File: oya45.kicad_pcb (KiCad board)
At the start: 2 copper layers, 190.5 x 95.2 mm, 108 parts, among them U1 ProMicro

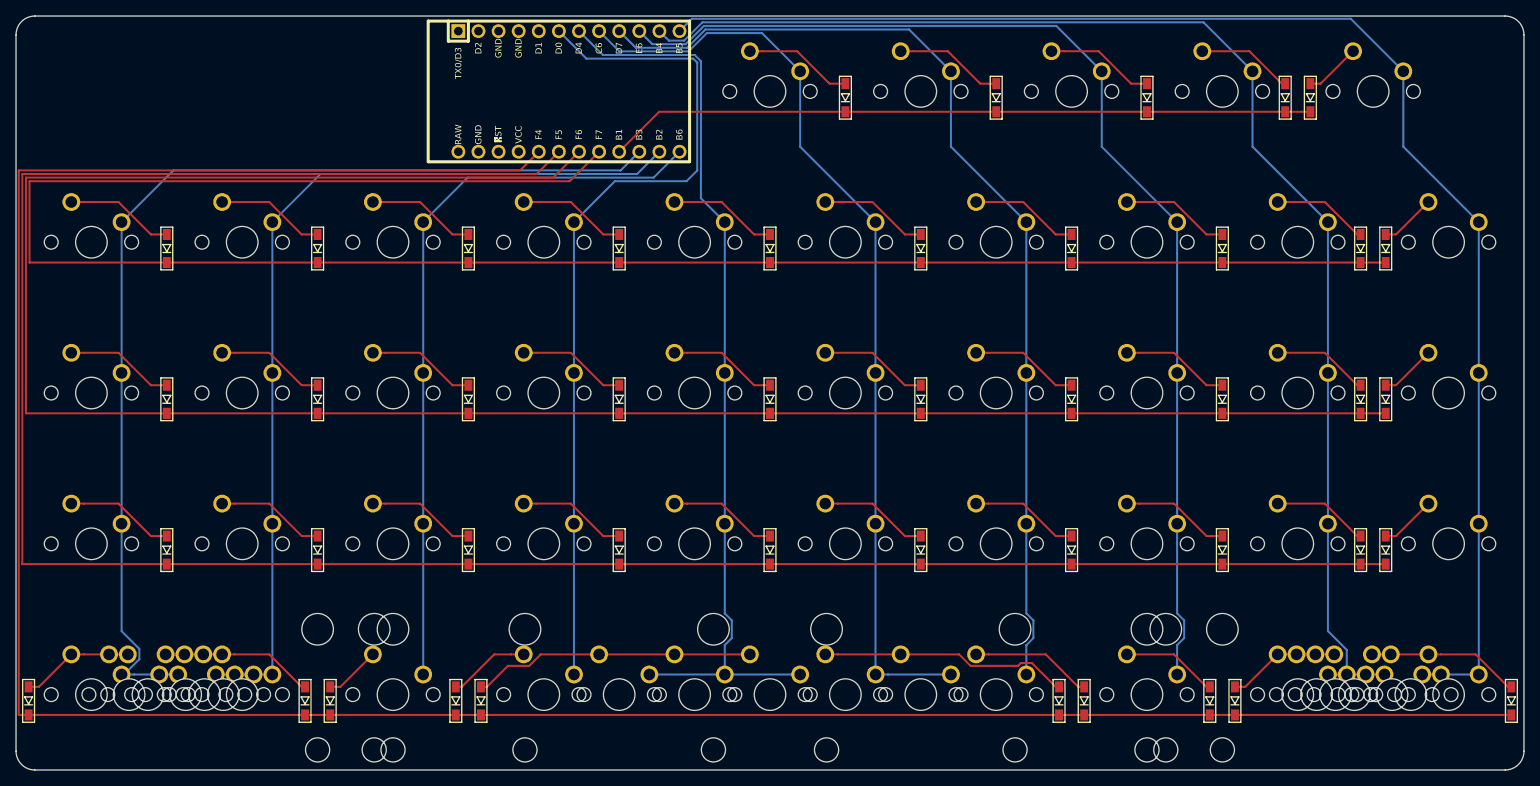
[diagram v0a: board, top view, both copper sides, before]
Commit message: added ground fill
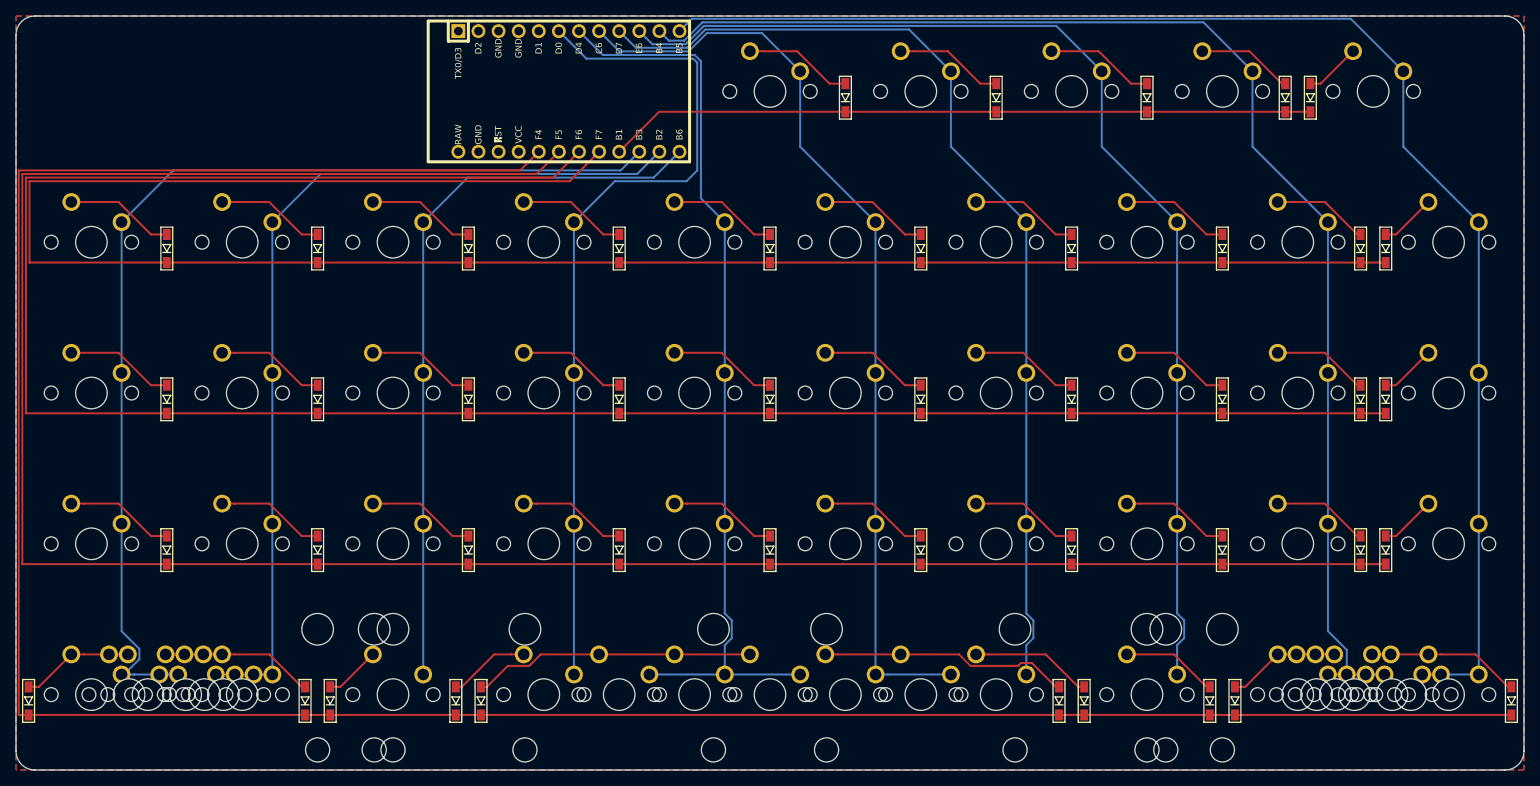
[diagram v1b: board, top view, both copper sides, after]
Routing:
- added copper zone on B.Cu, net (none)
- added copper zone on F.Cu, net (none)
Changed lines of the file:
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@@
   (segment (start 216.23974 28.91474) (end 133.01026 28.91474) (width 0.254) (layer B.Cu) (net 60))
   (segment (start 232.41 111.76) (end 225.26625 111.76) (width 0.254) (layer B.Cu) (net 60))
+  (zone (net 0) (net_name "") (layer F.Cu) (hatch edge 0.508)
+    (connect_pads (clearance 0.508))
+    (min_thickness 0.254)
+    (fill yes (arc_segments 32) (thermal_gap 0.508) (thermal_bridge_width 0.508))
+    (polygon
+      (pts
+        (xy 47.625 28.575) (xy 238.125 28.575) (xy 238.125 123.825) (xy 47.625 123.825)
+      )
+    )
+  )
+  (zone (net 0) (net_name "") (layer B.Cu) (hatch edge 0.508)
+    (connect_pads (clearance 0.508))
+    (min_thickness 0.254)
+    (fill yes (arc_segments 32) (thermal_gap 0.508) (thermal_bridge_width 0.508))
+    (polygon
+      (pts
+        (xy 47.625 28.575) (xy 238.125 28.575) (xy 238.125 123.825) (xy 47.625 123.825)
+      )
+    )
+  )
 )
